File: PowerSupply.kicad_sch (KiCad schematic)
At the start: 15 parts, among them U4 UM1750S-00

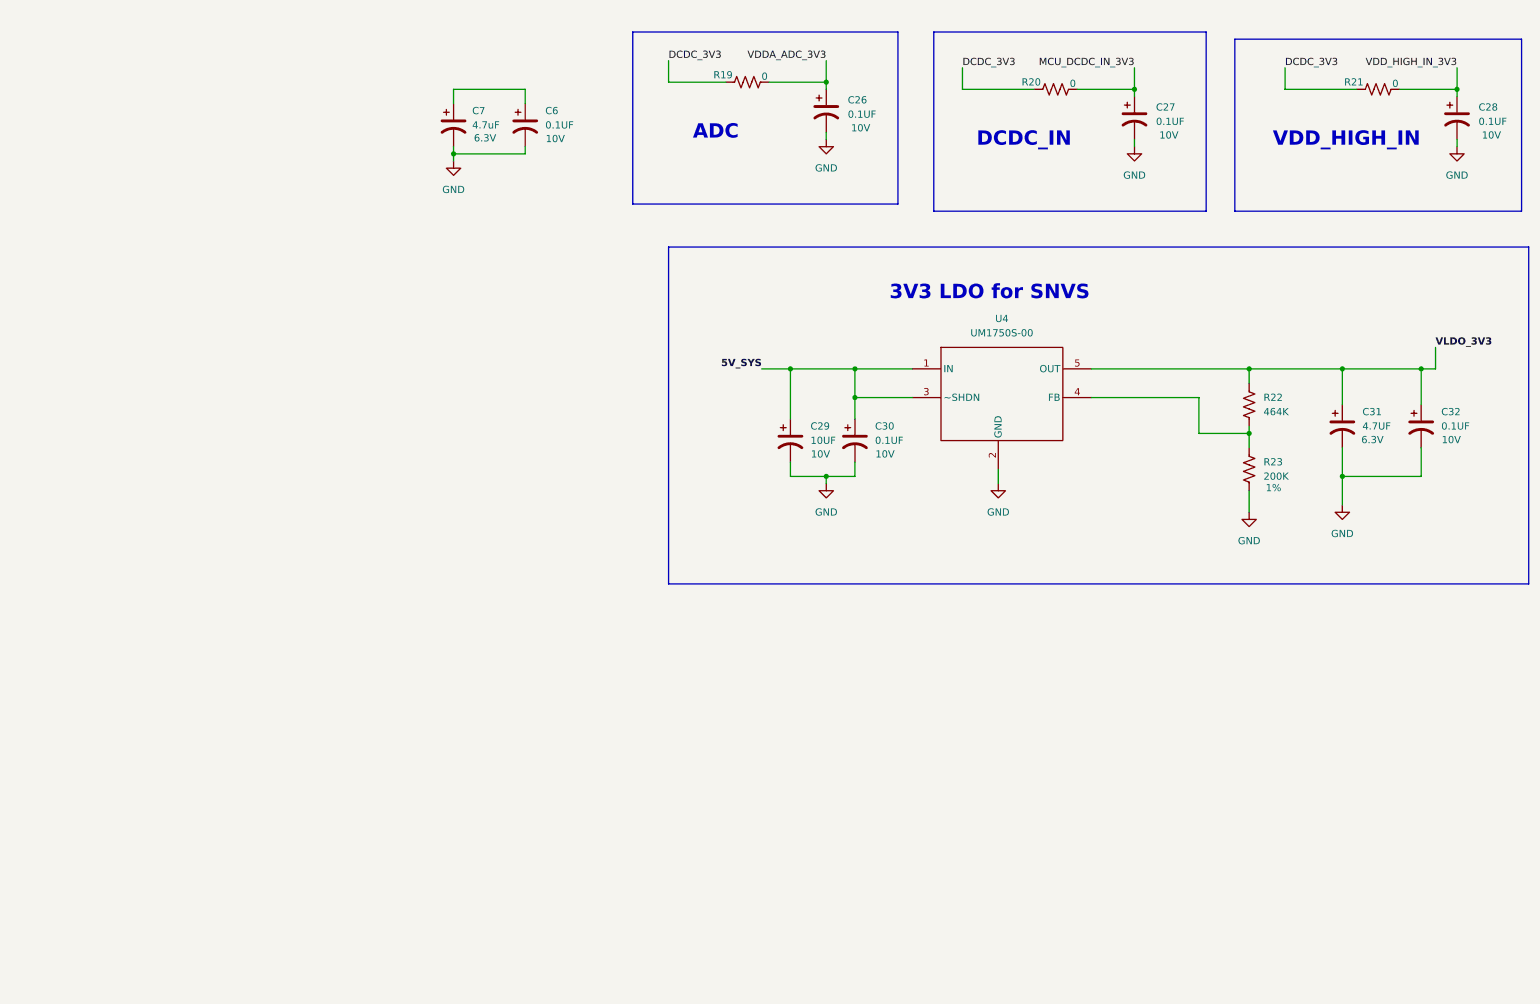
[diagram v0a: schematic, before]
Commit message: sebelum pemeriksaan terkahir
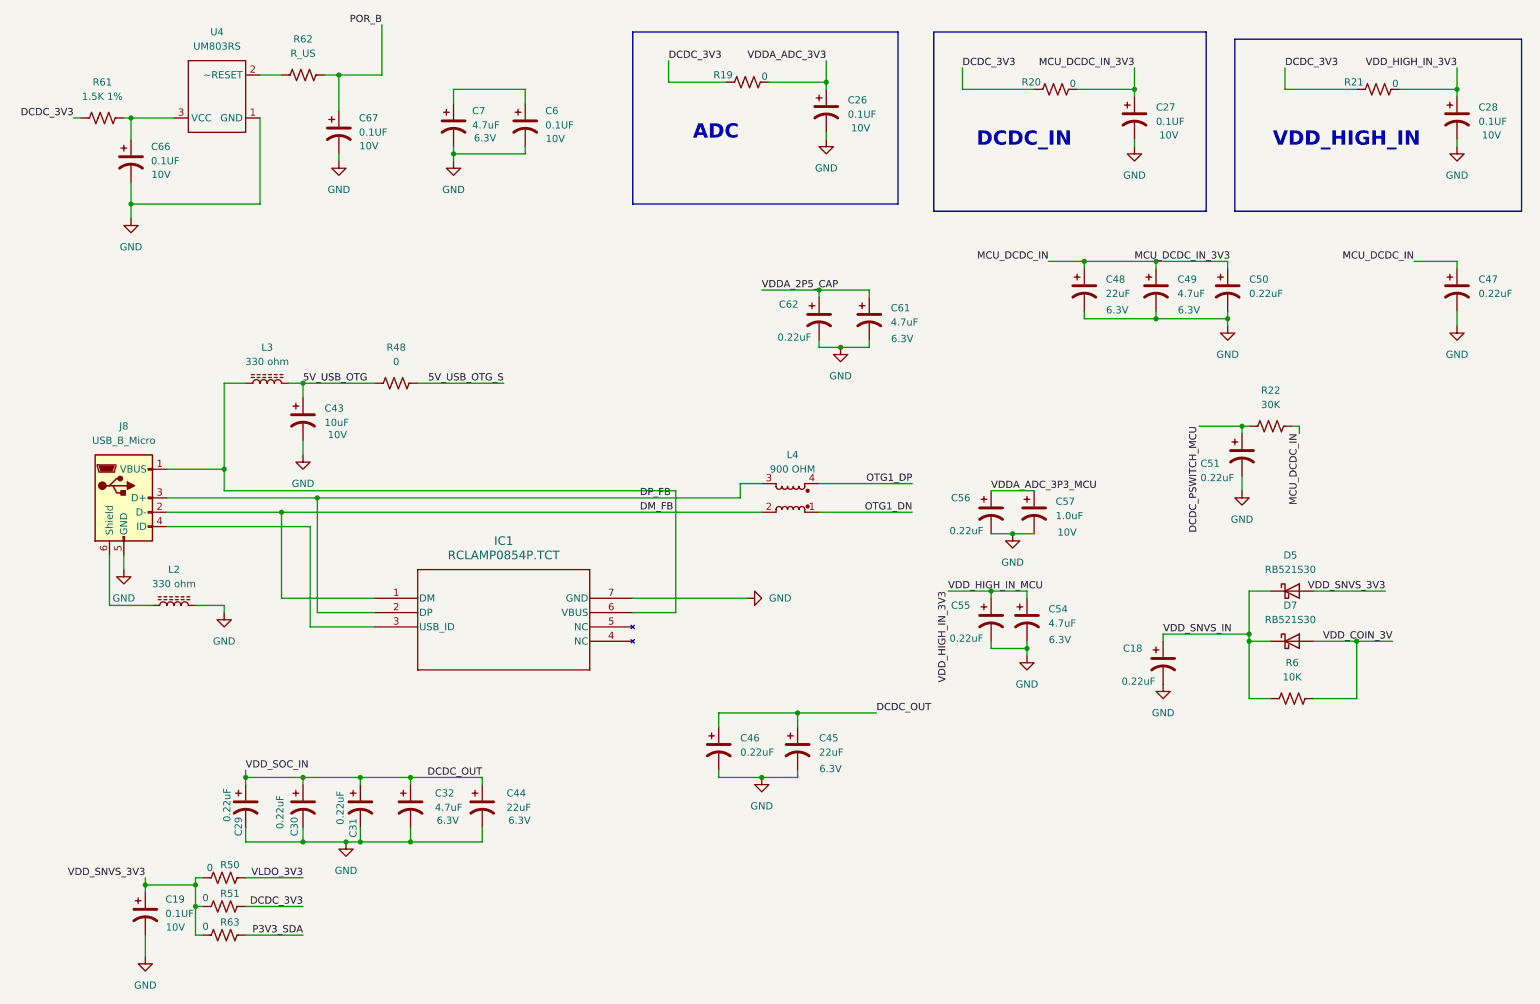
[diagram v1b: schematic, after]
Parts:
- removed R23: 200K, symbol Device:R_US
- removed U4: UM1750S-00, symbol qris_iot:UM1750S-00
- added C18, C46, C47, C50, C51, C55, C56, C62: 0.22uF, symbol Device:C_Polarized_US
- added C19, C66, C67: 0.1UF, symbol Device:C_Polarized_US
- added C43: 10uF, symbol Device:C_Polarized_US
- added C44, C45, C48: 22uF, symbol Device:C_Polarized_US
- added C49, C54, C61: 4.7uF, symbol Device:C_Polarized_US
- added C57: 1.0uF, symbol Device:C_Polarized_US
- added D5, D7: RB521S30, symbol Device:D_Schottky
- added IC1: RCLAMP0854P.TCT, UFDFN06_1P6X1P6_SEM, symbol tvs:RCLAMP0854P.TCT
- added J8: USB_B_Micro, symbol Connector:USB_B_Micro
- added L2, L3: 330 ohm, symbol Device:L_Ferrite
- added L4: 900 OHM, symbol Device:L_Coupled_1243
- added R48, R50, R51, R63: 0, symbol Device:R_US
- added R6: 10K, symbol Device:R_US
- added R61: 1.5K 1%, symbol Device:R_US
- added R62: R_US, symbol Device:R_US
- added U4: UM803RS, symbol tvs:UM803RS
- C29: value 10UF -> 0.22uF; Value2 10V -> (none)
- C30: value 0.1UF -> 0.22uF; Value2 10V -> (none)
- C31: value 4.7UF -> 0.22uF; Value2 6.3V -> (none)
- C32: value 0.1UF -> 4.7uF; Value2 10V -> 6.3V
- R22: value 464K -> 30K
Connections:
- net DCDC_3V3: now also R51.2, R61.1
- net GND: now also C18.2, C19.2, C43.2, C44.2, C45.2, C46.2, C47.2, C48.2, C49.2, C50.2, C51.2, C54.2, C55.2, C56.2, C57.2, C61.2, C62.2, C66.2, C67.2, IC1.7 (GND), J8.5 (GND), L2.2, U4.1 (GND)
- net VDD_HIGH_IN_3V3: now also C54.1, C55.1
- net VLDO_3V3: now also R50.2; no longer C31.1, C32.1, R22.2
- net DCDC_PSWITCH_MCU: now reaches R22.1
- net DCDC_PSWITCH_MCU: now also C51.1
- net 5V_SYS renamed DCDC_OUT
- net DCDC_OUT: now also C31.1, C32.1, C44.1, C45.1, C46.1
- net MCU_DCDC_IN_3V3 renamed MCU_DCDC_IN
- net MCU_DCDC_IN: now also R22.2, C47.1, C48.1, C49.1, C50.1
- new net: J8.6 (Shield), L2.1
- new net: IC1.3 (USB_ID), J8.4 (ID)
- new net: IC1.6 (VBUS), J8.1 (VBUS), L3.1
- new net: R62.1, U4.2 (~RESET)
- new net: C66.1, R61.2, U4.3 (VCC)
- new net 5V_USB_OTG: C43.1, L3.2, R48.1
- new net 5V_USB_OTG_S: R48.2
- new net DM_FB: IC1.1 (DM), J8.2 (D-), L4.2
- new net DP_FB: IC1.2 (DP), J8.3 (D+), L4.3
- new net OTG1_DN: L4.1
- new net OTG1_DP: L4.4
- new net P3V3_SDA: R63.2
- new net POR_B: C67.1, R62.2
- new net VDDA_2P5_CAP: C61.1, C62.1
- new net VDDA_ADC_3P3_MCU: C56.1, C57.1
- new net VDD_COIN_3V: D7.2 (A), R6.2
- new net VDD_SNVS_3V3: C19.1, D5.2 (A), R50.1, R51.1, R63.1
- new net VDD_SNVS_IN: C18.1, D5.1 (K), D7.1 (K), R6.1
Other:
- note removed: "3V3 LDO for SNVS"
